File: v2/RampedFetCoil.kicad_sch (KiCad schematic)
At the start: 151 parts, among them J1 FTSH-105-01-L-DV-K-P, J2 36503305, J3 703W-00_52, J4 Conn_01x01, J5 Conn_01x01, J6 Conn_01x01, J7 Conn_01x01, K2 G5Q-1, M1 Fan_CPU_4pin, Q1 C3M0120100K, Q2 C3M0120100K, Q3 C3M0120100K, Q4 C3M0120100K, Q5 T2N7002AK, Q6 T2N7002AK, Q7 T2N7002AK, T1 7492540200, U1 STM32G431KBTx, U11 UCC21520DW, U13 MGJ1D121505VMC-R7, U14 UCC21520DW, U15 MGJ1D121505VMC-R7, U16 MGJ1D121505VMC-R7, U2 74LVC1G14, U3 AP3928S-13, U4 CSTNE8M00G550000R0, U5 NCP1117-3.3_SOT223, U6 MCP9700T-E/TT, U7 74LVC1G14, U8 MGJ1D121505VMC-R7, U9 IF D95-T

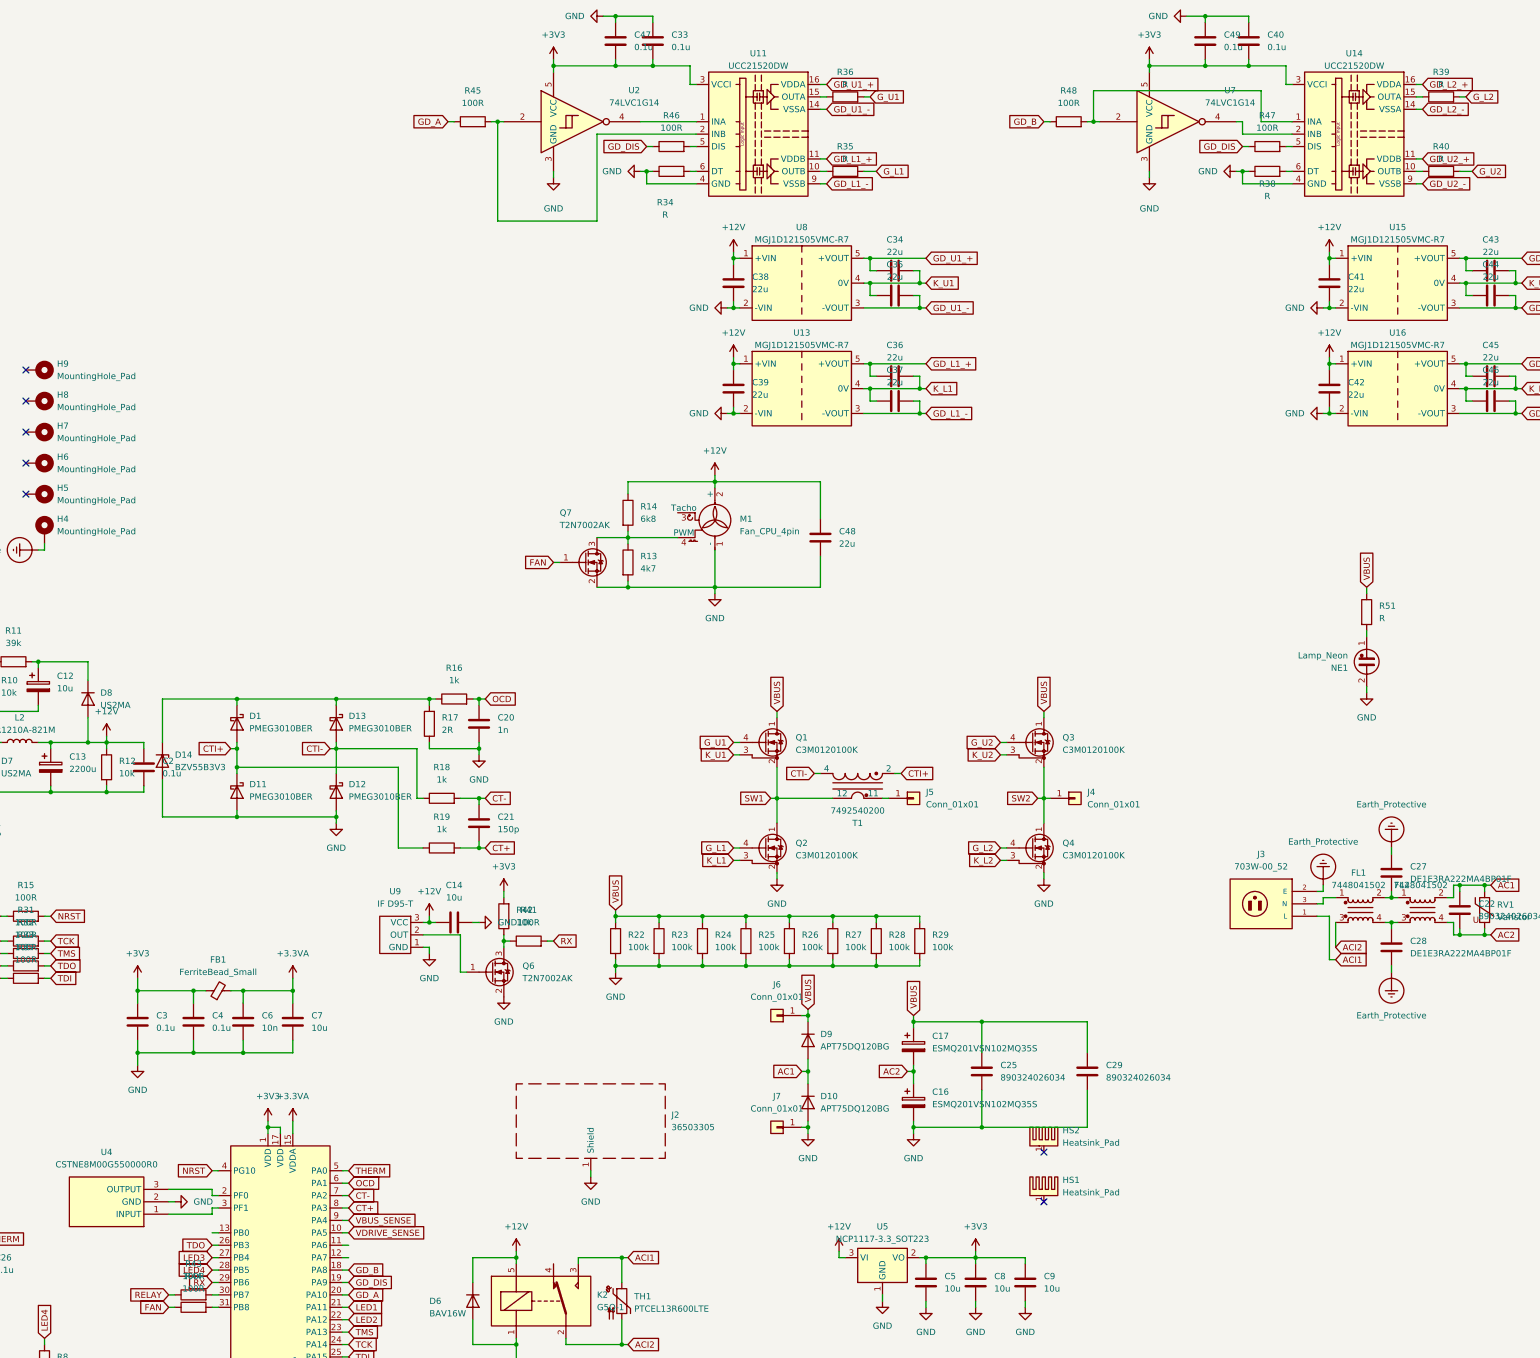
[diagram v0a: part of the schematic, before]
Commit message: sicswap 2
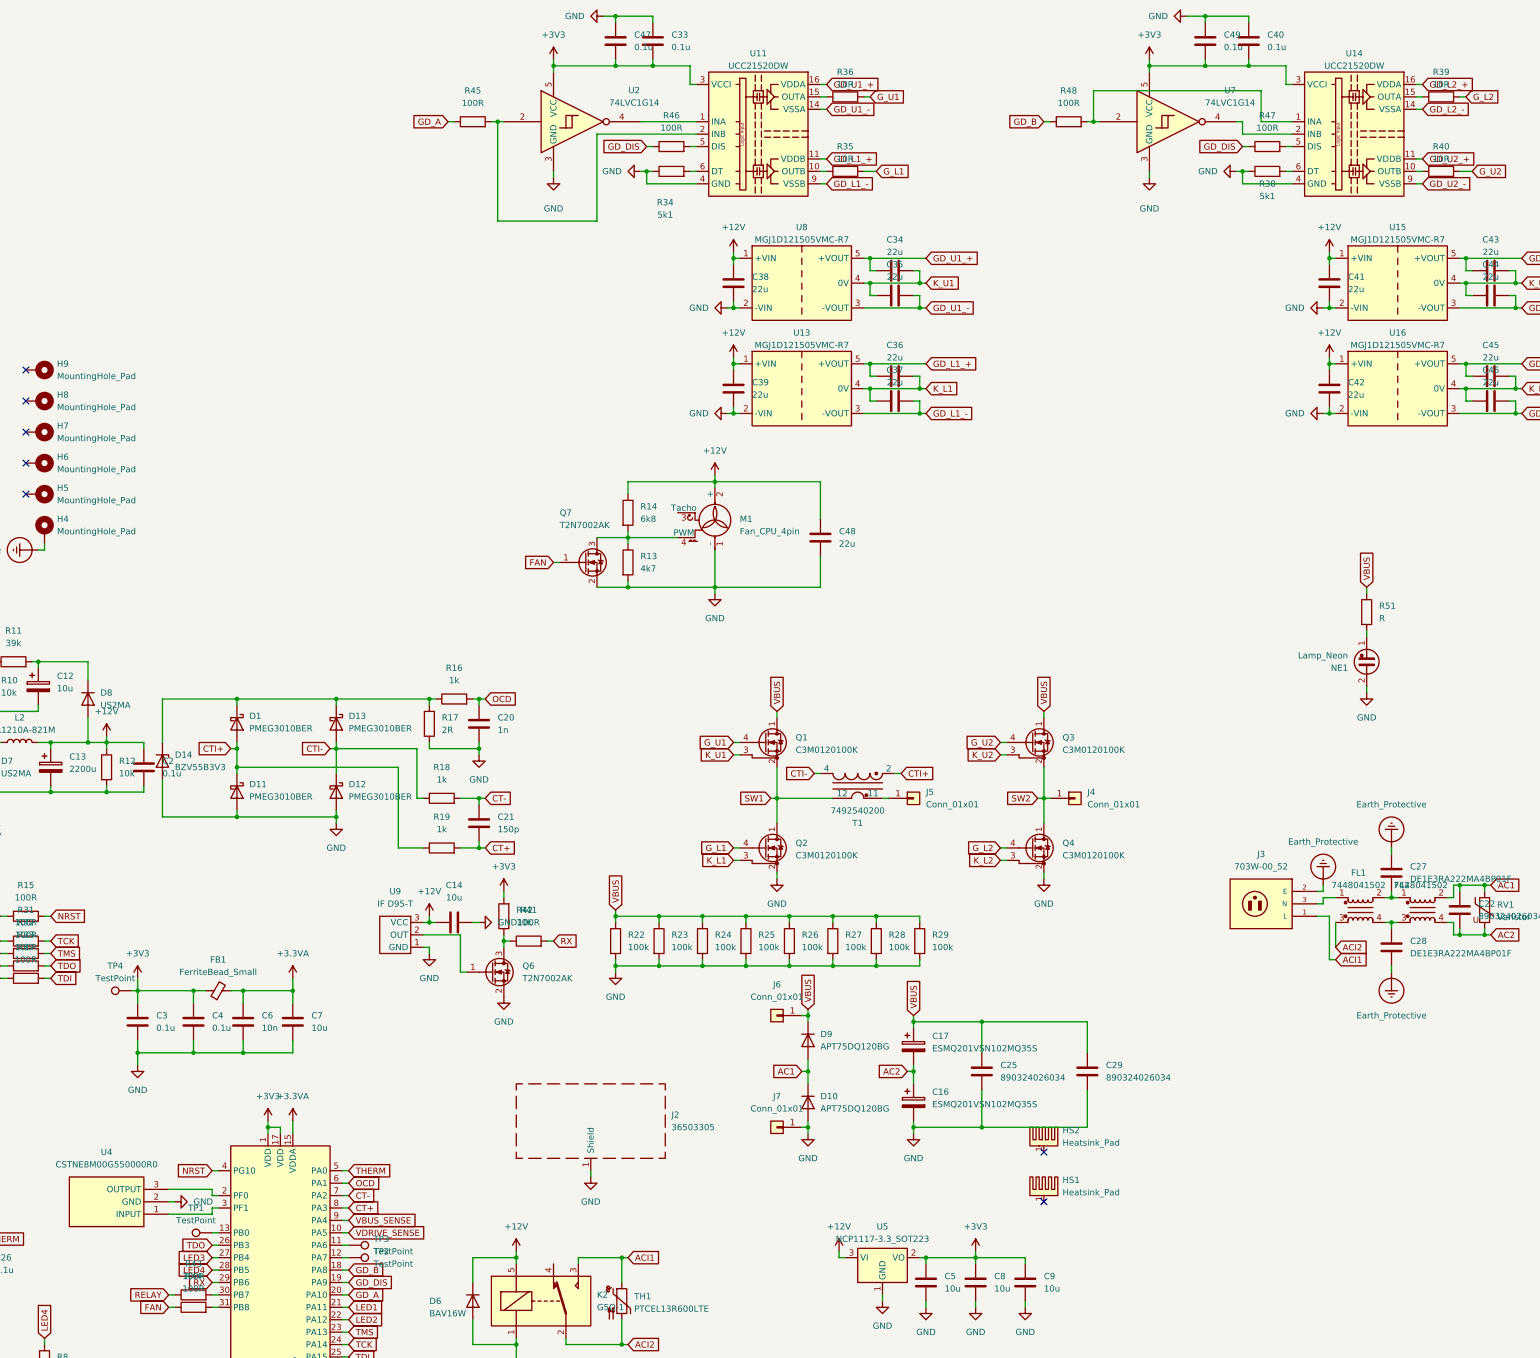
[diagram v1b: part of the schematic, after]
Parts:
- added TP1, TP2, TP3, TP4: TestPoint, TestPoint:TestPoint_Pad_1.5x1.5mm, symbol Connector:TestPoint
- R34, R38: value R -> 5k1
- R35, R36, R39, R40: value R -> 10R
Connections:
- net +3V3: now also TP4.1
- net at U1.11 (PA6): now also TP3.1
- net at U1.12 (PA7): now also TP2.1
- net at U1.13 (PB0): now also TP1.1
